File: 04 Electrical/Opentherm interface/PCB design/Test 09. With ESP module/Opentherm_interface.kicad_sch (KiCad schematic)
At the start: 20 parts, among them J2 Boiler, Q1 MMBT2907A, U3 EL357N-G, U4 EL357N-G

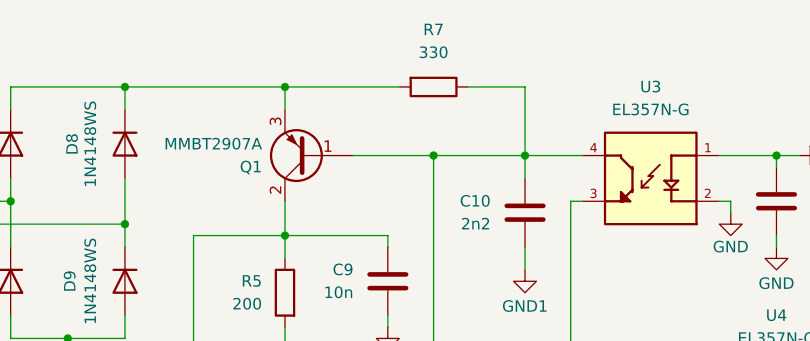
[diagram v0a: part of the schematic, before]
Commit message: Schematic update
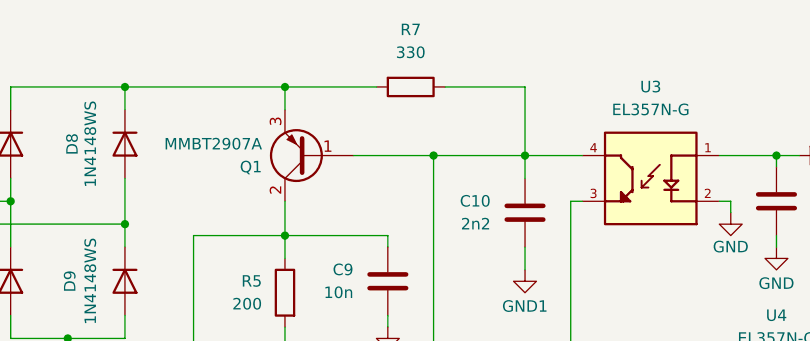
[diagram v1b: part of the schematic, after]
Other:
- moved on the sheet: R7
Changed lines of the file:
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@@
 	(wire
 		(pts
-			(xy 140.97 72.39) (xy 128.27 72.39)
+			(xy 138.43 72.39) (xy 128.27 72.39)
 		)
 		(stroke
@@
 	(wire
 		(pts
-			(xy 148.59 72.39) (xy 154.94 72.39)
+			(xy 146.05 72.39) (xy 154.94 72.39)
 		)
 		(stroke
@@
 	(symbol
 		(lib_id "Device:R")
-		(at 144.78 72.39 270)
+		(at 142.24 72.39 270)
 		(unit 1)
 		(exclude_from_sim no)
@@
 		(fields_autoplaced yes)
 		(property "Reference" "R7"
-			(at 144.78 66.04 90)
+			(at 142.24 66.04 90)
 			(effects
 				(font
@@
 		)
 		(property "Value" "330"
-			(at 144.78 68.58 90)
+			(at 142.24 68.58 90)
 			(effects
 				(font
@@
 		)
 		(property "Footprint" "Resistor_SMD:R_0805_2012Metric"
-			(at 144.78 70.612 90)
+			(at 142.24 70.612 90)
 			(effects
 				(font
@@
 		)
 		(property "Datasheet" "~"
-			(at 144.78 72.39 0)
+			(at 142.24 72.39 0)
 			(effects
 				(font
@@
 		)
 		(property "Description" "Resistor"
-			(at 144.78 72.39 0)
+			(at 142.24 72.39 0)
 			(effects
 				(font
@@
 		)
 		(property "LCSC Part # " "C17630"
-			(at 144.78 72.39 0)
-			(effects
-				(font
+			(at 142.24 72.39 0)
+			(effects
+				(font
